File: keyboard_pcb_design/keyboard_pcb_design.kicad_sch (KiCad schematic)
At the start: 39 parts, among them J1 USB_C_Receptacle_USB2.0_14P, SW1 Switch, SW2 Switch, SW3 Switch, SW4 Switch, SW5 Switch, U1 SC09147, U2 NCP1117-3.3_SOT223, U3 MX25L3233FM2I-08Q, U4 SMF05CT1G, X1 ABM8-272-T3

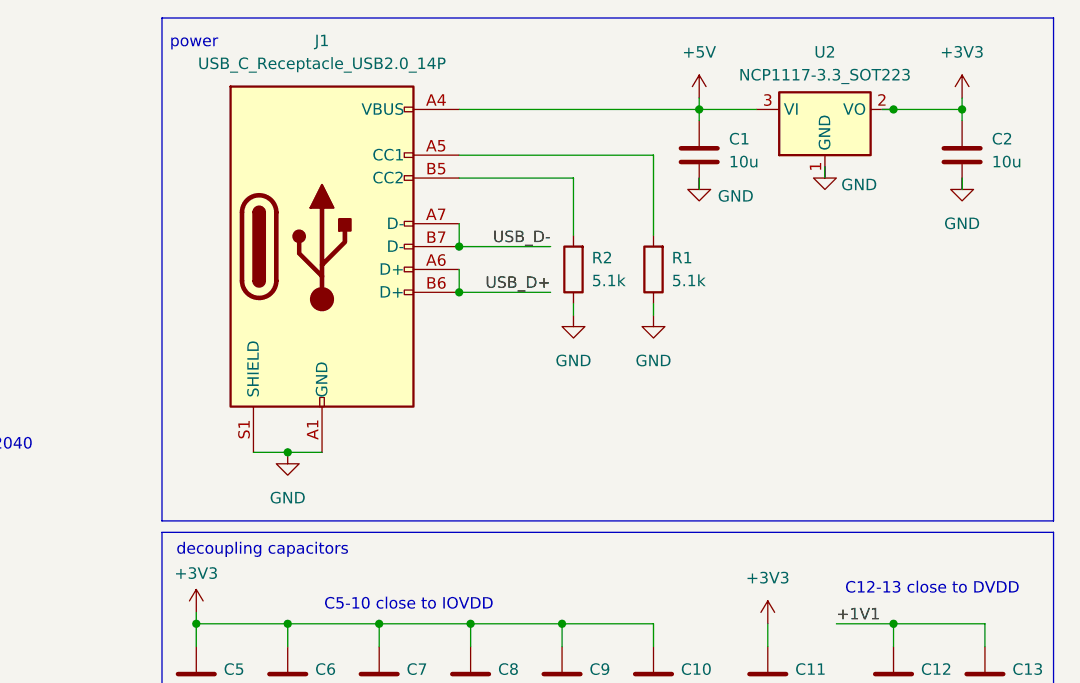
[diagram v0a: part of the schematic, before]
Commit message: saved changes
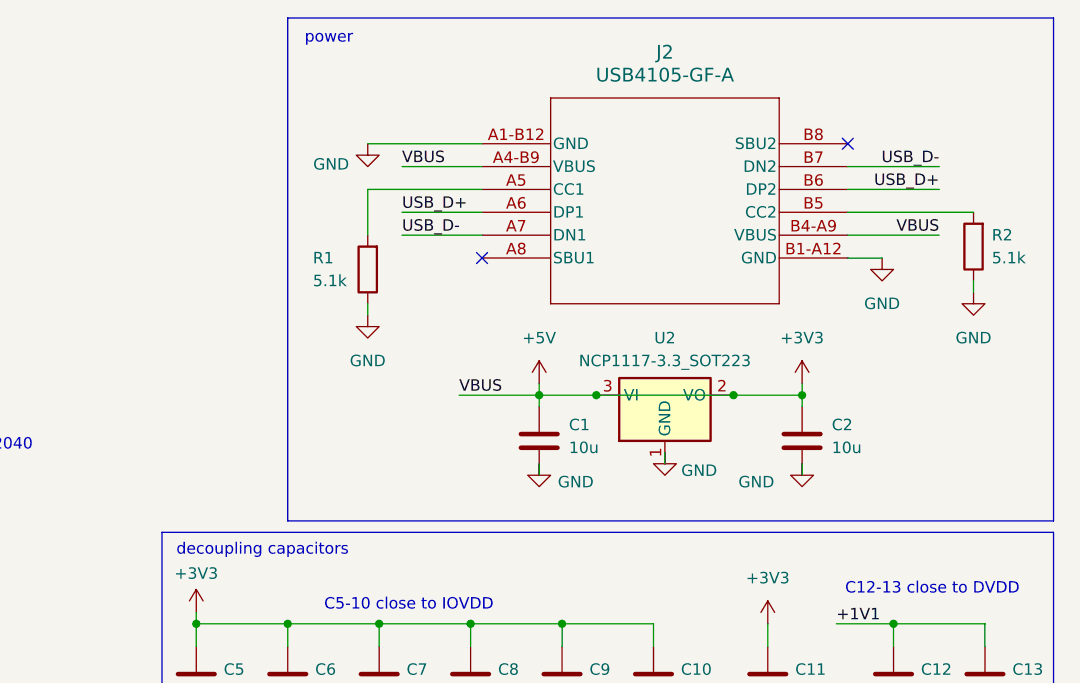
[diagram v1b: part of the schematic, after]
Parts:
- removed J1: USB_C_Receptacle_USB2.0_14P, symbol Connector:USB_C_Receptacle_USB2.0_14P
- added J2: USB4105-GF-A, keyboard_footprint:USB4105_GCT, symbol keyboard_library:USB4105-GF-A
- U4: footprint (none) -> keyboard_footprint:SOT65P210X110-6N
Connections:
- net +5V is gone; now on net +3V3: C1.1, U2.3 (VI), U4.4
- net +3V3: now also J2.A4-B9 (VBUS), J2.B4-A9 (VBUS)
- net GND: now also J2.A1-B12 (GND), J2.B1-A12 (GND)
- net USB_D+: now also J2.A6 (DP1), J2.B6 (DP2)
- net USB_D-: now also J2.A7 (DN1), J2.B7 (DN2)
- net at R1.2: now also J2.A5 (CC1)
- net at R2.2: now also J2.B5 (CC2)
- no-connect marks 1 -> 3
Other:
- moved on the sheet: C1, C2, R1, R2, U2
